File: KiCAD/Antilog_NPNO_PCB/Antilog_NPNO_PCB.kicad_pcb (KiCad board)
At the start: 2 copper layers, 38 parts, among them J1 PWR_IN, J2 TP_GND, J3 Couarse, J4 Modulation, J5 Master_Out, J6 I_REF, J7 I_Sink, Q1 2SC1815, Q2 2SC1815, U1 TL072

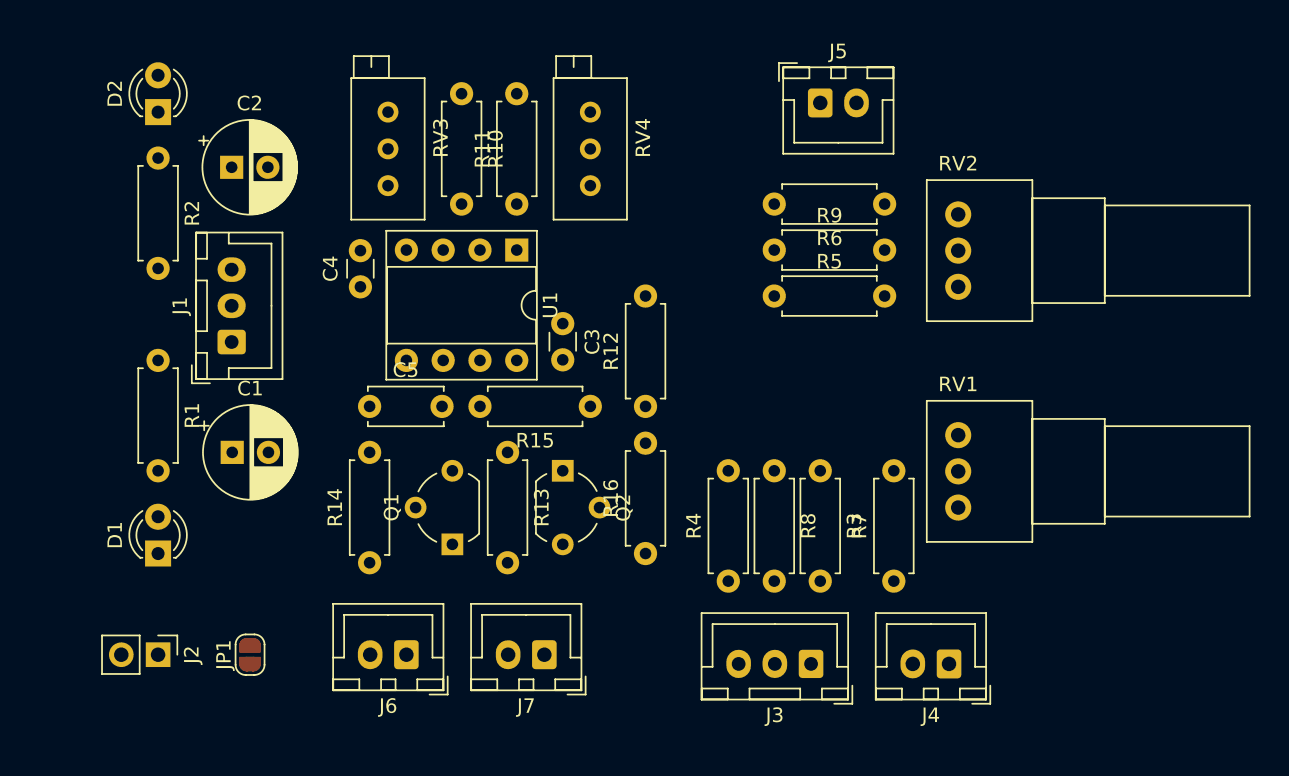
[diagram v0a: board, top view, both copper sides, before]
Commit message: implementation Test
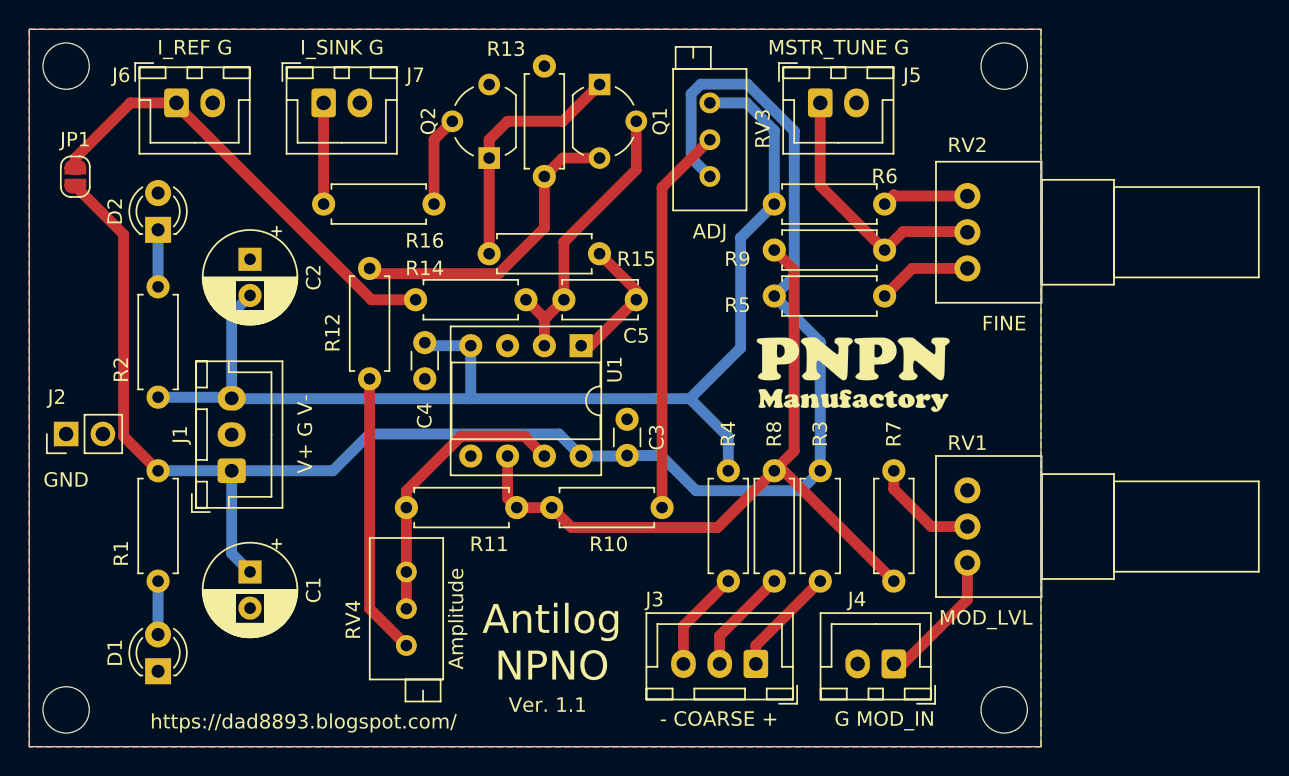
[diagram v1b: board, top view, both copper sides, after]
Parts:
- added G***: LOGO, myfootprint:Silk_PNPN_Manufactory_600dpi, F.Cu at (158.5, 93.4)
- added H1: MountingHole, MountingHole:MountingHole_3.2mm_M3, F.Cu at (104.1, 72.4)
- added H2: MountingHole, MountingHole:MountingHole_3.2mm_M3, F.Cu at (168.9, 72.4)
- added H3: MountingHole, MountingHole:MountingHole_3.2mm_M3, F.Cu at (104.1, 116.8)
- added H4: MountingHole, MountingHole:MountingHole_3.2mm_M3, F.Cu at (168.9, 116.8)
- moved J6 41.3 mm to (111.8, 74.9), turned to 0 degrees
- moved J7 41.0 mm to (121.9, 74.9), turned to 0 degrees
- moved JP1 35.1 mm to (104.8, 80.0), turned to 270 degrees
- moved Q1 33.3 mm to (141.0, 73.7), turned to 270 degrees
- moved R16 32.8 mm to (121.9, 81.9), turned to 0 degrees
- moved R10 31.8 mm to (145.3, 102.9), turned to 180 degrees
- moved RV4 29.5 mm to (127.6, 107.3), turned to 90 degrees
- moved R11 22.3 mm to (127.6, 102.9), turned to 0 degrees
- moved RV3 22.2 mm to (148.6, 80.0)
- moved Q2 22.2 mm to (133.3, 78.7), turned to 90 degrees
- moved R12 21.3 mm to (125.1, 86.4), turned to 270 degrees
- moved C5 19.8 mm to (143.5, 88.5), turned to 180 degrees
- moved R13 19.2 mm to (137.2, 80.0), turned to 90 degrees
- moved R14 18.4 mm to (128.3, 88.5), turned to 0 degrees
- moved J2 16.5 mm to (104.1, 97.8), turned to 90 degrees
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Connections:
- U1 pad 1: Net-(R11-Pad1) -> Net-(C5-Pad1)
- U1 pad 2: Net-(R10-Pad2) -> Net-(C5-Pad2)
- U1 pad 6: Net-(C5-Pad2) -> Net-(R10-Pad2)
- U1 pad 7: Net-(C5-Pad1) -> Net-(R11-Pad1)
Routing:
- net +12V: track 0.00 -> 118.8 mm
- net -12V: track 0.00 -> 83.6 mm
- net Net-(R10-Pad2): track 0.00 -> 51.6 mm
- net Net-(J6-Pad1): track 0.00 -> 31.4 mm
- net Net-(R10-Pad1): track 0.00 -> 26.8 mm
- net Net-(Q1-Pad3): track 0.00 -> 21.4 mm
- net Net-(C5-Pad2): track 0.00 -> 20.0 mm
- net Net-(R11-Pad1): track 0.00 -> 19.8 mm
- net Net-(R12-Pad2): track 0.00 -> 19.5 mm
- net Net-(J5-Pad1): track 0.00 -> 18.3 mm
- net Net-(Q1-Pad1): track 0.00 -> 17.7 mm
- net Net-(J4-Pad1): track 0.00 -> 9.46 mm
- net Net-(C5-Pad1): track 0.00 -> 9.35 mm
- net Net-(J3-Pad1): track 0.00 -> 7.56 mm
- net Net-(R7-Pad2): track 0.00 -> 7.42 mm
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- added copper zone on B.Cu, net GND
- added copper zone on F.Cu, net GND
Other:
- board outline added: 69.8 x 49.5 mm
- board text added: "- COARSE +"
- board text added: "ADJ"
- board text added: "Amplitude"
- board text added: "Antilog NPNO"
- board text added: "FINE"
- board text added: "G MOD_IN"
- board text added: "GND"
- board text added: "I_REF G"
- board text added: "I_SINK G"
- board text added: "MOD_LVL"
- board text added: "MSTR_TUNE G"
- board text added: "V+ G V-"
- board text added: "Ver. 1.1"
- board text added: "https://dad8893.blogspot.com/"
